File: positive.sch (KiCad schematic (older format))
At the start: 25 parts, among them U3 FOD8316, U6 Transformer_2P_2S

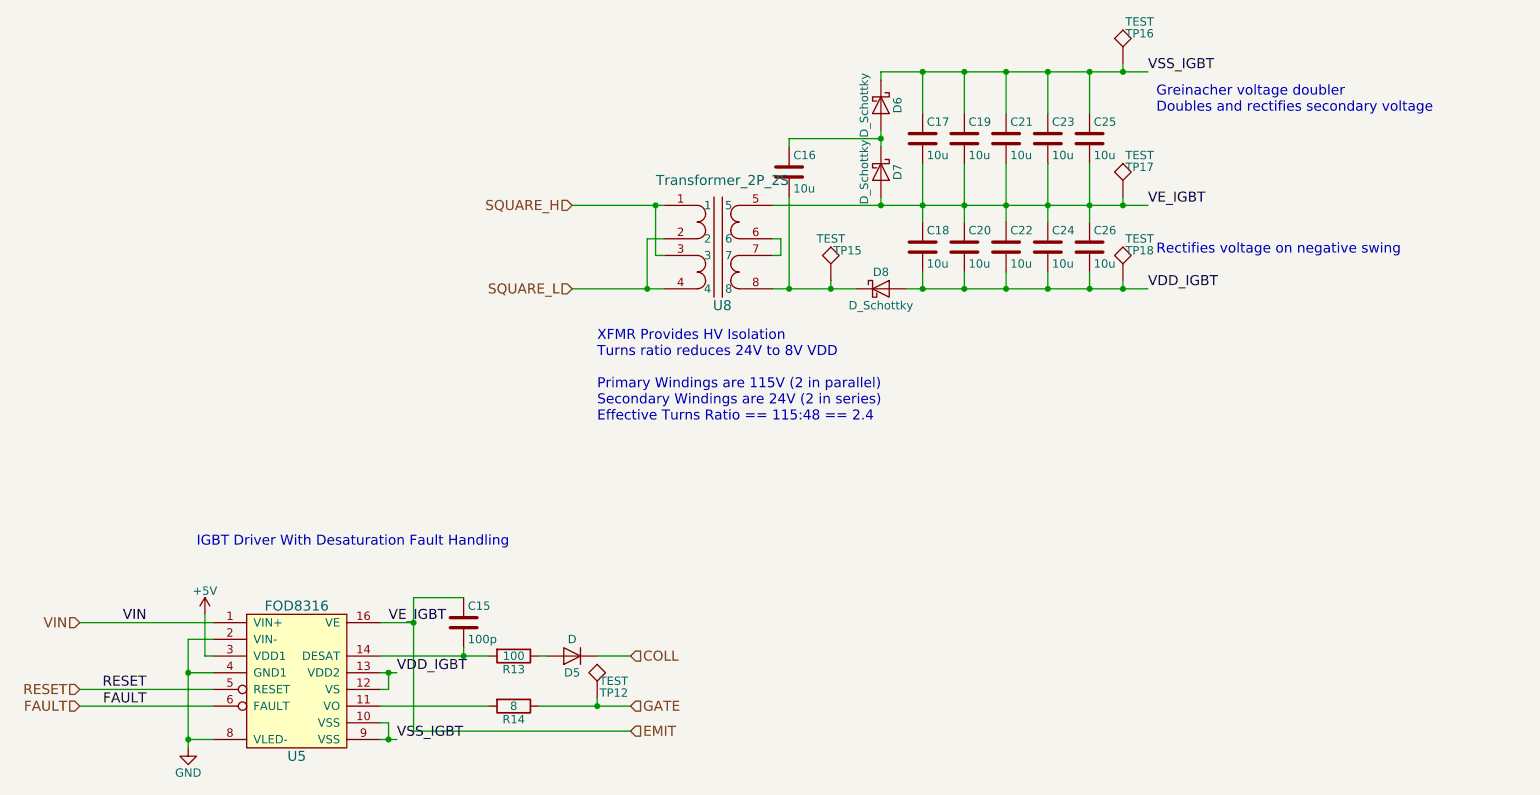
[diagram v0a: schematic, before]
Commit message: Changed 555 timer configuration.
555 timer was not behaving correctly. Added resistor to out for timing and increased resistor to 5V to mostly open circuit (in steady state).

Added extra coupling capacitor for control voltage.
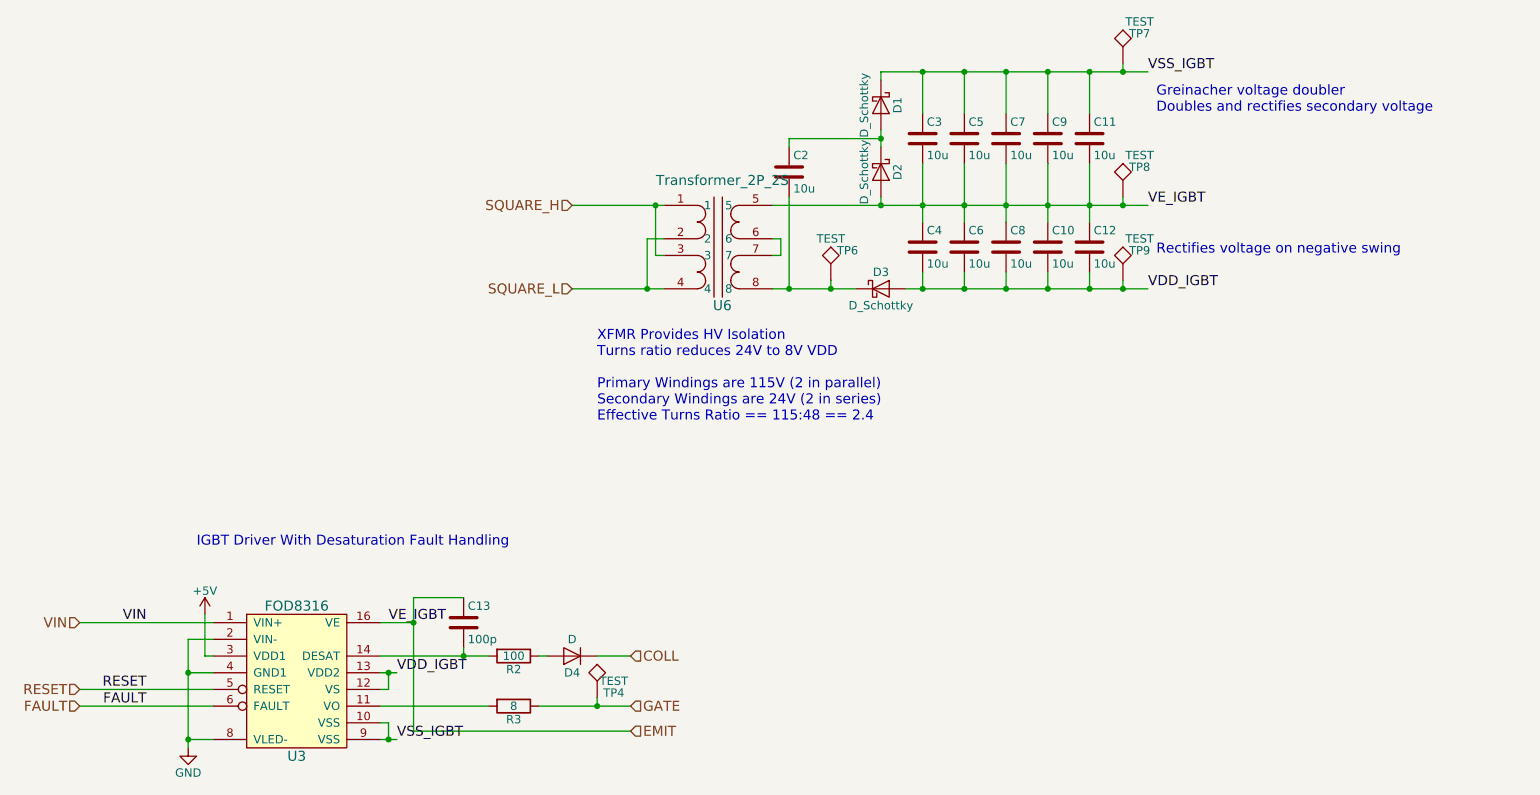
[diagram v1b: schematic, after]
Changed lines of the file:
@@
 AR Path="/5AD96A61/5AD97D83" Ref="C4"  Part="1"
 AR Path="/5ADA6656/5AD97D83" Ref="C18"  Part="1"
-F 0 "C18" H 6325 2400 50  0000 L CNN
+F 0 "C4" H 6325 2400 50  0000 L CNN
 F 1 "10u" H 6325 2200 50  0000 L CNN
 F 2 "Capacitors_SMD:C_1206_HandSoldering" H 6338 2150 50  0001 C CNN
@@
 AR Path="/5AD96A61/5AD97D8A" Ref="C3"  Part="1"
 AR Path="/5ADA6656/5AD97D8A" Ref="C17"  Part="1"
-F 0 "C17" H 6325 1750 50  0000 L CNN
+F 0 "C3" H 6325 1750 50  0000 L CNN
 F 1 "10u" H 6325 1550 50  0000 L CNN
 F 2 "Capacitors_SMD:C_1206_HandSoldering" H 6338 1500 50  0001 C CNN
@@
 AR Path="/5AD96A61/5AD97D91" Ref="C2"  Part="1"
 AR Path="/5ADA6656/5AD97D91" Ref="C16"  Part="1"
-F 0 "C16" H 5525 1950 50  0000 L CNN
+F 0 "C2" H 5525 1950 50  0000 L CNN
 F 1 "10u" H 5525 1750 50  0000 L CNN
 F 2 "Capacitors_SMD:C_1206_HandSoldering" H 5538 1700 50  0001 C CNN
@@
 AR Path="/5AD96A61/5AD97D98" Ref="D2"  Part="1"
 AR Path="/5ADA6656/5AD97D98" Ref="D7"  Part="1"
-F 0 "D7" H 6050 1950 50  0000 C CNN
+F 0 "D2" H 6050 1950 50  0000 C CNN
 F 1 "D_Schottky" H 6050 1750 50  0000 C CNN
 F 2 "Diodes_SMD:D_SOD-123F" H 6050 1850 50  0001 C CNN
@@
 AR Path="/5AD96A61/5AD97D9F" Ref="D1"  Part="1"
 AR Path="/5ADA6656/5AD97D9F" Ref="D6"  Part="1"
-F 0 "D6" H 6050 1550 50  0000 C CNN
+F 0 "D1" H 6050 1550 50  0000 C CNN
 F 1 "D_Schottky" H 6050 1350 50  0000 C CNN
 F 2 "Diodes_SMD:D_SOD-123F" H 6050 1450 50  0001 C CNN
@@
 AR Path="/5AD96A61/5AD97DA6" Ref="D3"  Part="1"
 AR Path="/5ADA6656/5AD97DA6" Ref="D8"  Part="1"
-F 0 "D8" H 6050 2650 50  0000 C CNN
+F 0 "D3" H 6050 2650 50  0000 C CNN
 F 1 "D_Schottky" H 6050 2450 50  0000 C CNN
 F 2 "Diodes_SMD:D_SOD-123F" H 6050 2550 50  0001 C CNN
@@
 AR Path="/5AD96A61/5AD97DE9" Ref="C5"  Part="1"
 AR Path="/5ADA6656/5AD97DE9" Ref="C19"  Part="1"
-F 0 "C19" H 6575 1750 50  0000 L CNN
+F 0 "C5" H 6575 1750 50  0000 L CNN
 F 1 "10u" H 6575 1550 50  0000 L CNN
 F 2 "Capacitors_SMD:C_1206_HandSoldering" H 6588 1500 50  0001 C CNN
@@
 AR Path="/5AD96A61/5AD97DF0" Ref="C7"  Part="1"
 AR Path="/5ADA6656/5AD97DF0" Ref="C21"  Part="1"
-F 0 "C21" H 6825 1750 50  0000 L CNN
+F 0 "C7" H 6825 1750 50  0000 L CNN
 F 1 "10u" H 6825 1550 50  0000 L CNN
 F 2 "Capacitors_SMD:C_1206_HandSoldering" H 6838 1500 50  0001 C CNN
@@
 AR Path="/5AD96A61/5AD97DF7" Ref="C9"  Part="1"
 AR Path="/5ADA6656/5AD97DF7" Ref="C23"  Part="1"
-F 0 "C23" H 7075 1750 50  0000 L CNN
+F 0 "C9" H 7075 1750 50  0000 L CNN
 F 1 "10u" H 7075 1550 50  0000 L CNN
 F 2 "Capacitors_SMD:C_1206_HandSoldering" H 7088 1500 50  0001 C CNN
@@
 AR Path="/5AD96A61/5AD97DFE" Ref="C11"  Part="1"
 AR Path="/5ADA6656/5AD97DFE" Ref="C25"  Part="1"
-F 0 "C25" H 7325 1750 50  0000 L CNN
+F 0 "C11" H 7325 1750 50  0000 L CNN
 F 1 "10u" H 7325 1550 50  0000 L CNN
 F 2 "Capacitors_SMD:C_1206_HandSoldering" H 7338 1500 50  0001 C CNN
@@
 AR Path="/5AD96A61/5AD97E05" Ref="C6"  Part="1"
 AR Path="/5ADA6656/5AD97E05" Ref="C20"  Part="1"
-F 0 "C20" H 6575 2400 50  0000 L CNN
+F 0 "C6" H 6575 2400 50  0000 L CNN
 F 1 "10u" H 6575 2200 50  0000 L CNN
 F 2 "Capacitors_SMD:C_1206_HandSoldering" H 6588 2150 50  0001 C CNN
@@
 AR Path="/5AD96A61/5AD97E0C" Ref="C8"  Part="1"
 AR Path="/5ADA6656/5AD97E0C" Ref="C22"  Part="1"
-F 0 "C22" H 6825 2400 50  0000 L CNN
+F 0 "C8" H 6825 2400 50  0000 L CNN
 F 1 "10u" H 6825 2200 50  0000 L CNN
 F 2 "Capacitors_SMD:C_1206_HandSoldering" H 6838 2150 50  0001 C CNN
@@
 AR Path="/5AD96A61/5AD97E13" Ref="C10"  Part="1"
 AR Path="/5ADA6656/5AD97E13" Ref="C24"  Part="1"
-F 0 "C24" H 7075 2400 50  0000 L CNN
+F 0 "C10" H 7075 2400 50  0000 L CNN
 F 1 "10u" H 7075 2200 50  0000 L CNN
 F 2 "Capacitors_SMD:C_1206_HandSoldering" H 7088 2150 50  0001 C CNN
@@
 AR Path="/5AD96A61/5AD97E1A" Ref="C12"  Part="1"
 AR Path="/5ADA6656/5AD97E1A" Ref="C26"  Part="1"
-F 0 "C26" H 7325 2400 50  0000 L CNN
+F 0 "C12" H 7325 2400 50  0000 L CNN
 F 1 "10u" H 7325 2200 50  0000 L CNN
 F 2 "Capacitors_SMD:C_1206_HandSoldering" H 7338 2150 50  0001 C CNN
@@
 AR Path="/5AD96A61/5AD97E37" Ref="TP6"  Part="1"
 AR Path="/5ADA6656/5AD97E37" Ref="TP15"  Part="1"
-F 0 "TP15" H 5850 2650 50  0000 C BNN
+F 0 "TP6" H 5850 2650 50  0000 C BNN
 F 1 "TEST" H 5750 2750 50  0000 C CNN
 F 2 "inverter-igbt-driver:TP RCT (0805)" H 5750 2500 50  0001 C CNN
@@
 AR Path="/5AD96A61/5AD97E3E" Ref="TP7"  Part="1"
 AR Path="/5ADA6656/5AD97E3E" Ref="TP16"  Part="1"
-F 0 "TP16" H 7600 1350 50  0000 C BNN
+F 0 "TP7" H 7600 1350 50  0000 C BNN
 F 1 "TEST" H 7600 1450 50  0000 C CNN
 F 2 "inverter-igbt-driver:TP RCT (0805)" H 7500 1200 50  0001 C CNN
@@
 AR Path="/5AD96A61/5AD97E45" Ref="TP8"  Part="1"
 AR Path="/5ADA6656/5AD97E45" Ref="TP17"  Part="1"
-F 0 "TP17" H 7600 2150 50  0000 C BNN
+F 0 "TP8" H 7600 2150 50  0000 C BNN
 F 1 "TEST" H 7600 2250 50  0000 C CNN
 F 2 "inverter-igbt-driver:TP RCT (0805)" H 7500 2000 50  0001 C CNN
@@
 AR Path="/5AD96A61/5AD97E4C" Ref="TP9"  Part="1"
 AR Path="/5ADA6656/5AD97E4C" Ref="TP18"  Part="1"
-F 0 "TP18" H 7600 2650 50  0000 C BNN
+F 0 "TP9" H 7600 2650 50  0000 C BNN
 F 1 "TEST" H 7600 2750 50  0000 C CNN
 F 2 "inverter-igbt-driver:TP RCT (0805)" H 7500 2500 50  0001 C CNN
@@
 AR Path="/5AD96A61/5AD97E53" Ref="U6"  Part="1"
 AR Path="/5ADA6656/5AD97E53" Ref="U8"  Part="1"
-F 0 "U8" H 5100 1650 60  0000 C CNN
+F 0 "U6" H 5100 1650 60  0000 C CNN
 F 1 "Transformer_2P_2S" H 5100 2400 60  0000 C CNN
 F 2 "inverter-igbt-driver:FS48-050-C2" H 5100 2150 60  0001 C CNN
@@
 AR Path="/5AD96A61/5AD9846B" Ref="U3"  Part="1"
 AR Path="/5ADA6656/5AD9846B" Ref="U5"  Part="1"
-F 0 "U5" H 2550 4450 60  0000 C CNN
+F 0 "U3" H 2550 4450 60  0000 C CNN
 F 1 "FOD8316" H 2550 5350 60  0000 C CNN
 F 2 "Housings_SOIC:SOIC-16W_7.5x10.3mm_Pitch1.27mm" H 2450 4950 60  0001 C CNN
@@
 AR Path="/5AD96A61/5AD98472" Ref="#PWR03"  Part="1"
 AR Path="/5ADA6656/5AD98472" Ref="#PWR05"  Part="1"
-F 0 "#PWR05" H 2000 4350 50  0001 C CNN
+F 0 "#PWR03" H 2000 4350 50  0001 C CNN
 F 1 "+5V" H 2000 4640 50  0000 C CNN
 F 2 "" H 2000 4500 50  0001 C CNN
@@
 AR Path="/5AD96A61/5AD98478" Ref="#PWR04"  Part="1"
 AR Path="/5ADA6656/5AD98478" Ref="#PWR06"  Part="1"
-F 0 "#PWR06" H 1900 5050 50  0001 C CNN
+F 0 "#PWR04" H 1900 5050 50  0001 C CNN
 F 1 "GND" H 1900 5150 50  0000 C CNN
 F 2 "" H 1900 5300 50  0001 C CNN
@@
 AR Path="/5AD96A61/5AD98484" Ref="R3"  Part="1"
 AR Path="/5ADA6656/5AD98484" Ref="R14"  Part="1"
-F 0 "R14" V 3930 5050 50  0000 C CNN
+F 0 "R3" V 3930 5050 50  0000 C CNN
 F 1 "8" V 3850 5050 50  0000 C CNN
 F 2 "Resistors_THT:R_Axial_DIN0207_L6.3mm_D2.5mm_P7.62mm_Horizontal" V 3780 5050 50  0001 C CNN
@@
 AR Path="/5AD96A61/5AD9848B" Ref="C13"  Part="1"
 AR Path="/5ADA6656/5AD9848B" Ref="C15"  Part="1"
-F 0 "C15" H 3575 4650 50  0000 L CNN
+F 0 "C13" H 3575 4650 50  0000 L CNN
 F 1 "100p" H 3575 4450 50  0000 L CNN
 F 2 "Capacitors_SMD:C_1206_HandSoldering" H 3588 4400 50  0001 C CNN
@@
 AR Path="/5AD96A61/5AD98492" Ref="R2"  Part="1"
 AR Path="/5ADA6656/5AD98492" Ref="R13"  Part="1"
-F 0 "R13" V 3930 4750 50  0000 C CNN
+F 0 "R2" V 3930 4750 50  0000 C CNN
 F 1 "100" V 3850 4750 50  0000 C CNN
 F 2 "Resistors_SMD:R_1206_HandSoldering" V 3780 4750 50  0001 C CNN
@@
 AR Path="/5AD96A61/5AD98499" Ref="D4"  Part="1"
 AR Path="/5ADA6656/5AD98499" Ref="D5"  Part="1"
-F 0 "D5" H 4200 4850 50  0000 C CNN
+F 0 "D4" H 4200 4850 50  0000 C CNN
 F 1 "D" H 4200 4650 50  0000 C CNN
 F 2 "inverter-igbt-driver:DO-214AC" H 4200 4750 50  0001 C CNN
@@
 AR Path="/5AD96A61/5AD984A1" Ref="TP4"  Part="1"
 AR Path="/5ADA6656/5AD984A1" Ref="TP12"  Part="1"
-F 0 "TP12" H 4450 5000 50  0000 C BNN
+F 0 "TP4" H 4450 5000 50  0000 C BNN
 F 1 "TEST" H 4450 5100 50  0000 C CNN
 F 2 "inverter-igbt-driver:TP RCT (0805)" H 4350 5000 50  0001 C CNN
